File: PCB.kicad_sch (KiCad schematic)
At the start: 17 parts, among them J1 Conector IR, J10 Conector ultrassonico esquerdo, J11 Conector ultrassonico central, J12 Conector ultrassonico direito, J13 Conector LED Extra, J14 Conector LORA, J15 ENCO_SW_Esq, J16 ENCO_SW_Dir, J18 LEDs, J2 Conector bluetooth, J3 Conector Acelerometro, J5 Conector servo, J7 Conector motor direito, J8 Conector motor esquerdo, J9 Conector alimentacao sensores

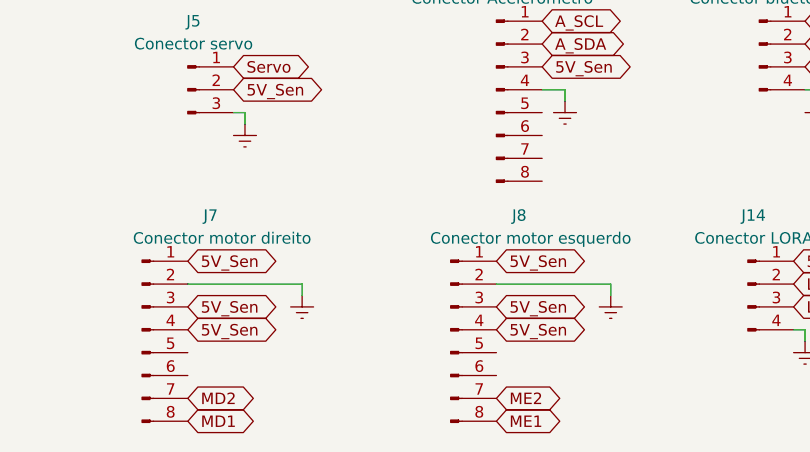
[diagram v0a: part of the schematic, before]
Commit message: feat: finalizacao da versao 2 da pcb
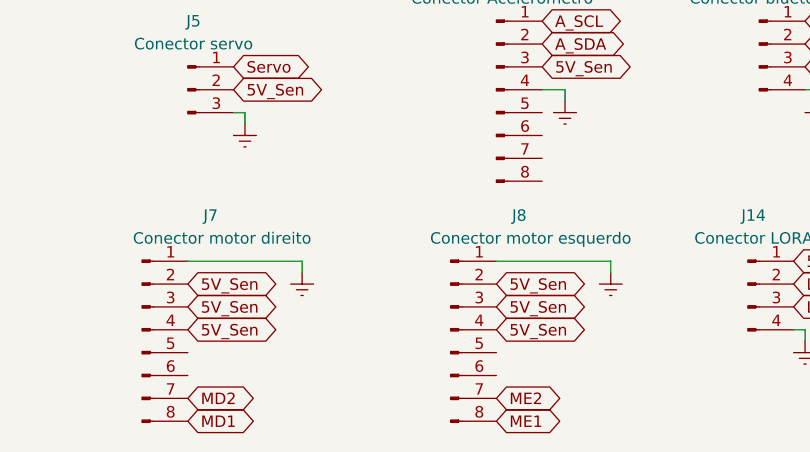
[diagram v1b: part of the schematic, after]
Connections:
- net 5V_Sen: now also J7.2 (Pin_2), J8.2 (Pin_2); no longer J7.1 (Pin_1), J8.1 (Pin_1)
- net Earth: now also J7.1 (Pin_1), J8.1 (Pin_1); no longer J7.2 (Pin_2), J8.2 (Pin_2)
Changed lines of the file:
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@@
 (kicad_sch (version 20230121) (generator eeschema)
   (paper "A4")
+  (wire (pts (xy 77.47 168.91) (xy 90.17 168.91))
+    (stroke (width 0) (type default))
+  )
   (wire (pts (xy 48.26 152.4) (xy 49.53 152.4))
     (stroke (width 0) (type default))
@@
     (stroke (width 0) (type default))
   )
-  (wire (pts (xy 90.17 171.45) (xy 90.17 172.72))
-    (stroke (width 0) (type default))
-  )
   (wire (pts (xy 193.04 146.05) (xy 194.31 146.05))
     (stroke (width 0) (type default))
@@
     (stroke (width 0) (type default))
   )
+  (wire (pts (xy 90.17 168.91) (xy 90.17 170.18))
+    (stroke (width 0) (type default))
+  )
+  (wire (pts (xy 55.88 168.91) (xy 55.88 170.18))
+    (stroke (width 0) (type default))
+  )
   (wire (pts (xy 138.43 166.37) (xy 152.4 166.37))
     (stroke (width 0) (type default))
@@
     (stroke (width 0) (type default))
   )
-  (wire (pts (xy 77.47 171.45) (xy 90.17 171.45))
+  (wire (pts (xy 43.18 168.91) (xy 55.88 168.91))
     (stroke (width 0) (type default))
   )
@@
     (stroke (width 0) (type default))
   )
-  (wire (pts (xy 43.18 171.45) (xy 55.88 171.45))
-    (stroke (width 0) (type default))
-  )
   (wire (pts (xy 166.37 158.75) (xy 167.64 158.75))
     (stroke (width 0) (type default))
   )
   (wire (pts (xy 111.76 176.53) (xy 111.76 177.8))
-    (stroke (width 0) (type default))
-  )
-  (wire (pts (xy 55.88 171.45) (xy 55.88 172.72))
     (stroke (width 0) (type default))
   )
@@
     )
   )
-  (global_label "5V_Sen" (shape bidirectional) (at 77.47 168.91 0) (fields_autoplaced)
-    (effects (font (size 1.27 1.27)) (justify left))
-    (property "Intersheetrefs" "${INTERSHEET_REFS}" (at 88.2793 168.91 0)
-      (effects (font (size 1.27 1.27)) (justify left) hide)
-    )
-  )
   (global_label "ECHO_2" (shape bidirectional) (at 138.43 161.29 0) (fields_autoplaced)
     (effects (font (size 1.27 1.27)) (justify left))
@@
     )
   )
-  (global_label "5V_Sen" (shape bidirectional) (at 43.18 168.91 0) (fields_autoplaced)
-    (effects (font (size 1.27 1.27)) (justify left))
-    (property "Intersheetrefs" "${INTERSHEET_REFS}" (at 53.9893 168.91 0)
+  (global_label "5V_Sen" (shape bidirectional) (at 43.18 171.45 0) (fields_autoplaced)
+    (effects (font (size 1.27 1.27)) (justify left))
+    (property "Intersheetrefs" "${INTERSHEET_REFS}" (at 53.9893 171.45 0)
       (effects (font (size 1.27 1.27)) (justify left) hide)
     )
@@
     (effects (font (size 1.27 1.27)) (justify left))
     (property "Intersheetrefs" "${INTERSHEET_REFS}" (at 148.816 144.78 0)
+      (effects (font (size 1.27 1.27)) (justify left) hide)
+    )
+  )
+  (global_label "5V_Sen" (shape bidirectional) (at 77.47 171.45 0) (fields_autoplaced)
+    (effects (font (size 1.27 1.27)) (justify left))
+    (property "Intersheetrefs" "${INTERSHEET_REFS}" (at 88.2793 171.45 0)
       (effects (font (size 1.27 1.27)) (justify left) hide)
     )
@@
     )
   )
+  (symbol (lib_id "power:Earth") (at 90.17 170.18 0) (unit 1)
+    (in_bom yes) (on_board yes) (dnp no) (fields_autoplaced)
+    (property "Reference" "#PWR04" (at 90.17 176.53 0)
+      (effects (font (size 1.27 1.27)) hide)
+    )
+    (property "Value" "Earth" (at 90.17 173.99 0)
+      (effects (font (size 1.27 1.27)) hide)
+    )
+    (property "Footprint" "" (at 90.17 170.18 0)
+      (effects (font (size 1.27 1.27)) hide)
+    )
+    (property "Datasheet" "~" (at 90.17 170.18 0)
+      (effects (font (size 1.27 1.27)) hide)
+    )
+    (pin "1")
+    (instances
+      (project "PCB"
+        (path "/b344186f-9059-49c5-a6f7-f90c862ad97f"
+          (reference "#PWR04") (unit 1)
+        )
+      )
+      (project "esquemaEletricoCarro"
+        (path "/e63e39d7-6ac0-4ffd-8aa3-1841a4541b55/980d7ea7-3ff9-498b-b91b-57f4a8ccee38"
+          (reference "#PWR08") (unit 1)
+        )
+      )
+    )
+  )
   (symbol (lib_id "Device:R") (at 203.2 143.51 90) (unit 1)
     (in_bom yes) (on_board yes) (dnp no) (fields_autoplaced)
@@
         (path "/e63e39d7-6ac0-4ffd-8aa3-1841a4541b55/ef1da815-5ae9-4f7a-859c-d7960e6acc1e"
           (reference "#PWR021") (unit 1)
-        )
-      )
-    )
-  )
-  (symbol (lib_id "power:Earth") (at 90.17 172.72 0) (unit 1)
-    (in_bom yes) (on_board yes) (dnp no) (fields_autoplaced)
-    (property "Reference" "#PWR04" (at 90.17 179.07 0)
-      (effects (font (size 1.27 1.27)) hide)
-    )
-    (property "Value" "Earth" (at 90.17 176.53 0)
-      (effects (font (size 1.27 1.27)) hide)
-    )
-    (property "Footprint" "" (at 90.17 172.72 0)
-      (effects (font (size 1.27 1.27)) hide)
-    )
-    (property "Datasheet" "~" (at 90.17 172.72 0)
-      (effects (font (size 1.27 1.27)) hide)
-    )
-    (pin "1")
-    (instances
-      (project "PCB"
-        (path "/b344186f-9059-49c5-a6f7-f90c862ad97f"
-          (reference "#PWR04") (unit 1)
-        )
-      )
-      (project "esquemaEletricoCarro"
-        (path "/e63e39d7-6ac0-4ffd-8aa3-1841a4541b55/980d7ea7-3ff9-498b-b91b-57f4a8ccee38"
-          (reference "#PWR08") (unit 1)
         )
       )
@@
     )
   )
-  (symbol (lib_id "power:Earth") (at 55.88 172.72 0) (unit 1)
-    (in_bom yes) (on_board yes) (dnp no) (fields_autoplaced)
-    (property "Reference" "#PWR010" (at 55.88 179.07 0)
-      (effects (font (size 1.27 1.27)) hide)
-    )
-    (property "Value" "Earth" (at 55.88 176.53 0)
-      (effects (font (size 1.27 1.27)) hide)
-    )
-    (property "Footprint" "" (at 55.88 172.72 0)
-      (effects (font (size 1.27 1.27)) hide)
-    )
-    (property "Datasheet" "~" (at 55.88 172.72 0)
-      (effects (font (size 1.27 1.27)) hide)
-    )
+  (symbol (lib_id "power:Earth") (at 55.88 170.18 0) (unit 1)
+    (in_bom yes) (on_board yes) (dnp no) (fields_autoplaced)
+    (property "Reference" "#PWR010" (at 55.88 176.53 0)
+      (effects (font (size 1.27 1.27)) hide)
+    )
+    (property "Value" "Earth" (at 55.88 173.99 0)
+      (effects (font (size 1.27 1.27)) hide)
+    )
+    (property "Footprint" "" (at 55.88 170.18 0)
+      (effects (font (size 1.27 1.27)) hide)
+    )
+    (property "Datasheet" "~" (at 55.88 170.18 0)
+      (effects (font (size 1.27 1.27)) hide)
+    )
